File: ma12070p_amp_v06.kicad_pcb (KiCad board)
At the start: 2 copper layers, 100.4 x 80.4 mm, 85 parts, among them U1 MAX16956, U2 MA12070P

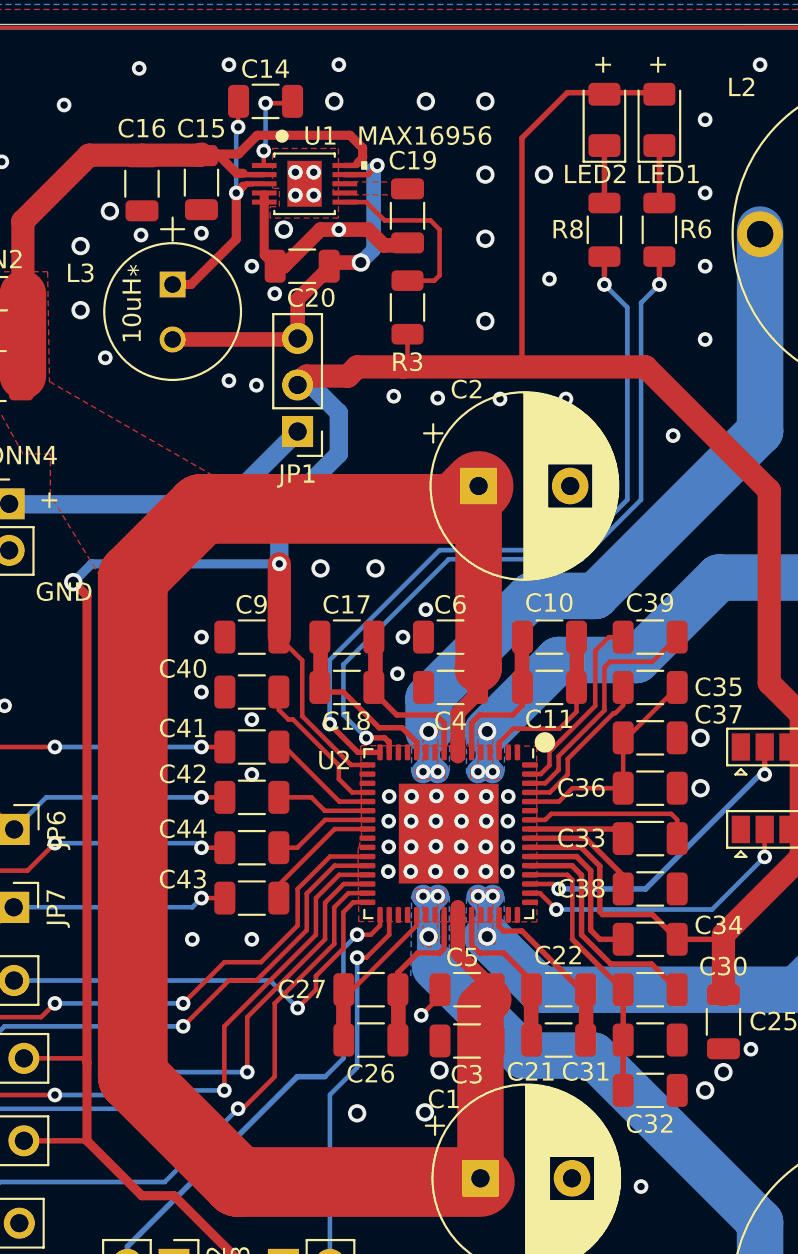
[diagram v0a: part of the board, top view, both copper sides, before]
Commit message: changes
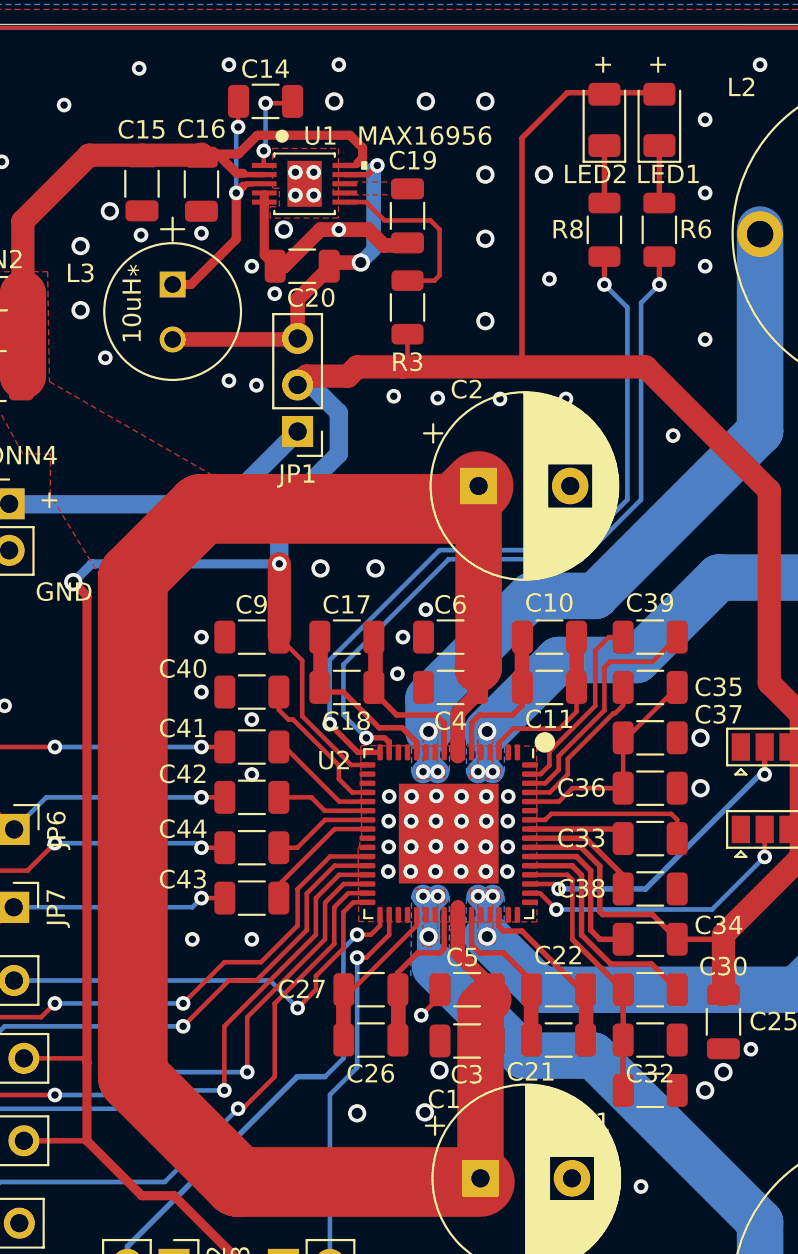
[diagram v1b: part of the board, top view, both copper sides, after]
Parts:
- moved C15 3.25 mm to (133.2, 52.5)
- moved C16 3.25 mm to (136.5, 52.5)
- moved C31 2.75 mm to (161.0, 102.0)
- moved C32 2.75 mm to (161.0, 99.2)
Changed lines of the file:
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@@
   )
   (footprint "Capacitor_SMD:C_1206_3216Metric" (layer "F.Cu")
-    (at 133.25 52.5 -90)
+    (at 136.5 52.525 -90)
     (descr "Capacitor SMD 1206 (3216 Metric), square (rectangular) end terminal, IPC_7351 nominal, (Body size source: IPC-SM-782 page 76, https://www.pcb-3d.com/wordpress/wp-content/uploads/ipc-sm-782a_amendment_1_and_2.pdf), generated with kicad-footprint-generator")
     (tags "capacitor")
@@
   )
   (footprint "Capacitor_SMD:C_1206_3216Metric" (layer "F.Cu")
-    (at 136.5 52.4375 -90)
+    (at 133.25 52.5 -90)
     (descr "Capacitor SMD 1206 (3216 Metric), square (rectangular) end terminal, IPC_7351 nominal, (Body size source: IPC-SM-782 page 76, https://www.pcb-3d.com/wordpress/wp-content/uploads/ipc-sm-782a_amendment_1_and_2.pdf), generated with kicad-footprint-generator")
     (tags "capacitor")
@@
   )
   (footprint "Capacitor_SMD:C_1206_3216Metric" (layer "F.Cu")
-    (at 161 99.25)
+    (at 161 102)
     (descr "Capacitor SMD 1206 (3216 Metric), square (rectangular) end terminal, IPC_7351 nominal, (Body size source: IPC-SM-782 page 76, https://www.pcb-3d.com/wordpress/wp-content/uploads/ipc-sm-782a_amendment_1_and_2.pdf), generated with kicad-footprint-generator")
     (tags "capacitor")
@@
   )
   (footprint "Capacitor_SMD:C_1206_3216Metric" (layer "F.Cu")
-    (at 161 102 180)
-    (descr "Capacitor SMD 1206 (3216 Metric), square (rectangular) end terminal, IPC_7351 nominal, (Body size source: IPC-SM-782 page 76, https://www.pcb-3d.com/wordpress/wp-content/uploads/ipc-sm-782a_amendment_1_and_2.pdf), generated with kicad-footprint-generator")
-    (tags "capacitor")
+    (at 161 99.25 180)
+    (descr "Capacitor SMD 1206 (3216 Metric), square (rectangular) end terminal, IPC_7351 nominal, (Body size source: IPC-SM-782 page 76, https://www.pcb-3d.com/wordpress/wp-content/uploads/ipc-sm-782a_amendment_1_and_2.pdf), generated with kicad-footprint-generator")
+    (tags "capacitor")
